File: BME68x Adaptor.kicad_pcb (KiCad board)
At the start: 2 copper layers, 20 x 20 mm, 7 parts, among them J1 Conn_01x06, U1 BME680

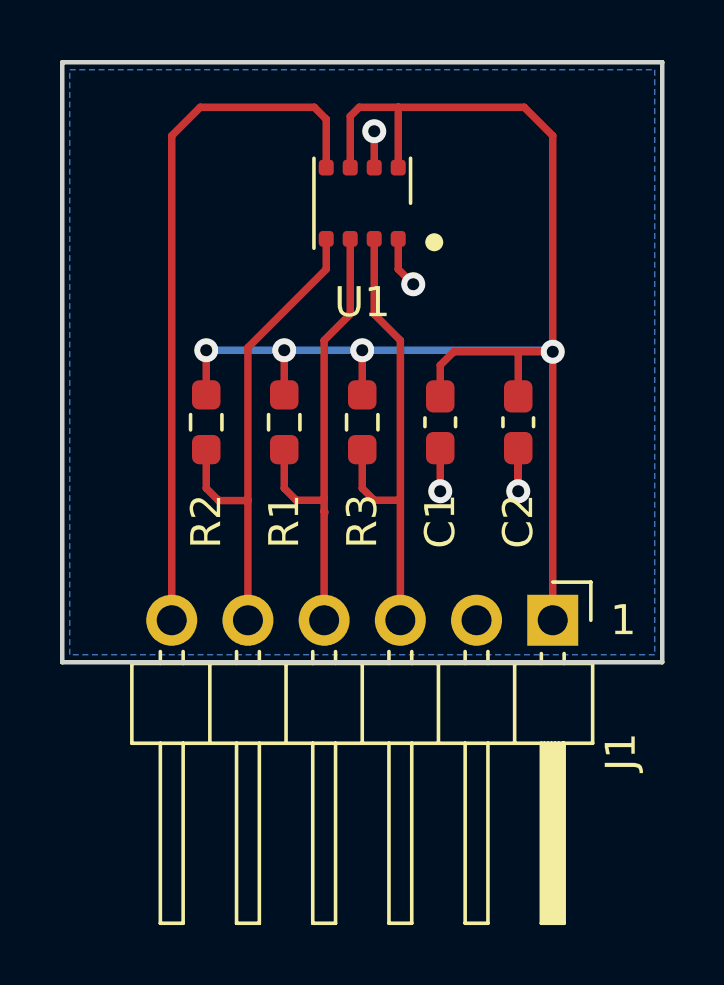
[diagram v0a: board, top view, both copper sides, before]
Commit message: Silkscreen improved
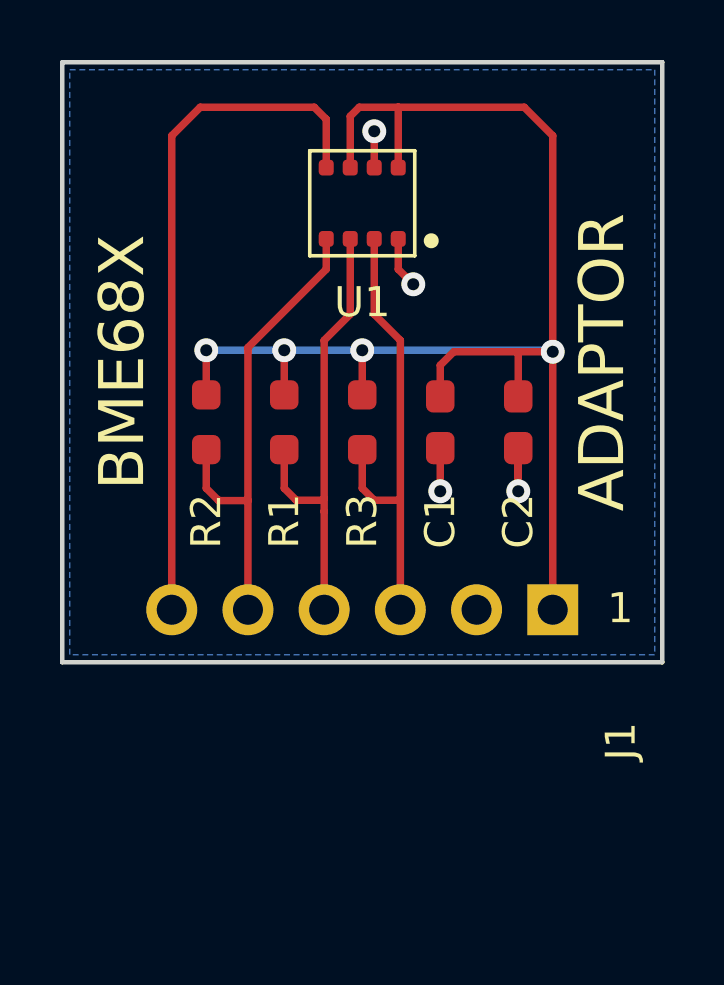
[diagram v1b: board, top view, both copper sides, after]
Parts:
- moved J1 0.35 mm to (146.3, 98.2)
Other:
- board text added: "ADAPTOR"
- board text added: "BME68X"
